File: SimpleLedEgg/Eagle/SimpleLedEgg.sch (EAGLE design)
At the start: 18 parts

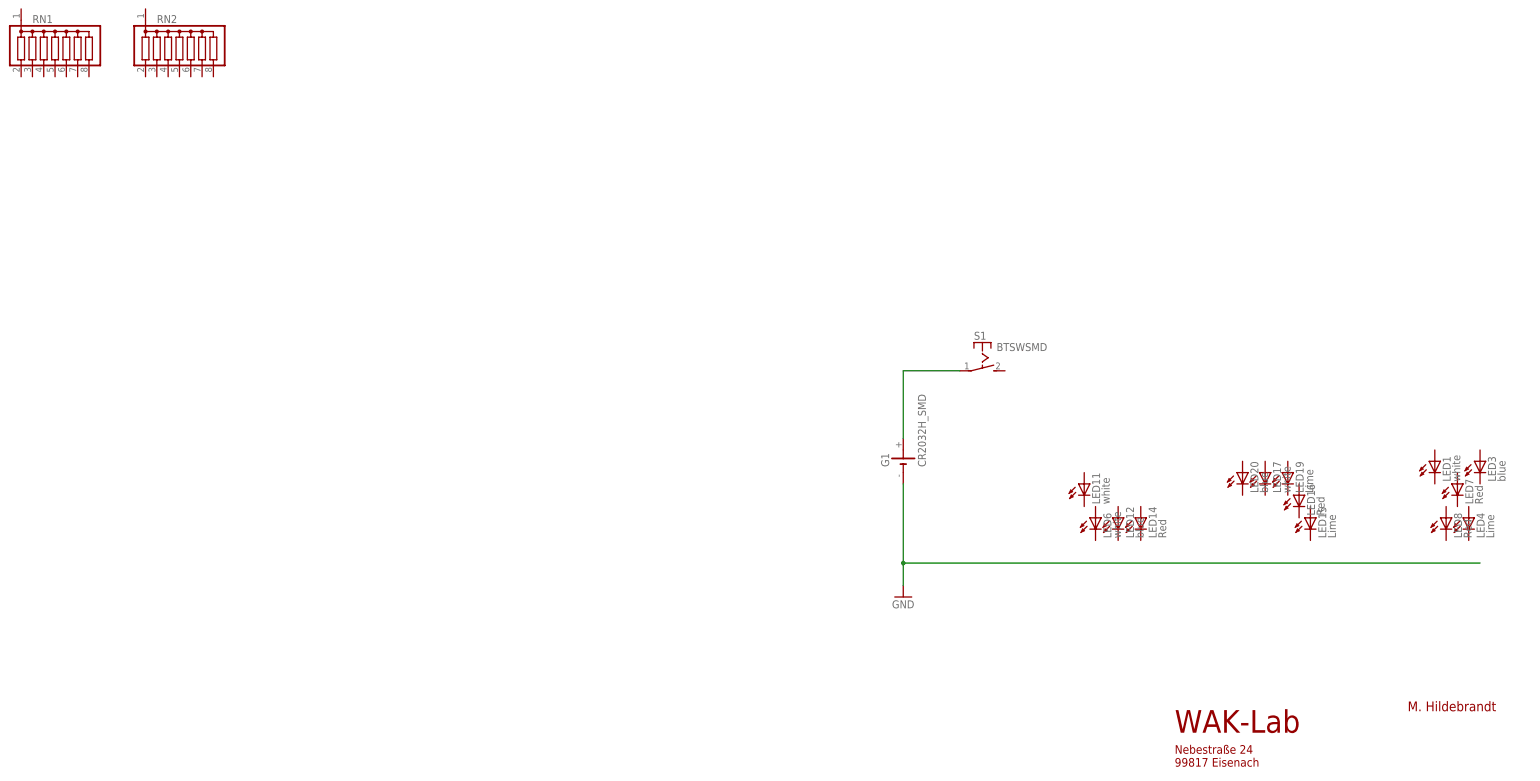
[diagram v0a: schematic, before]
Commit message: Gerber
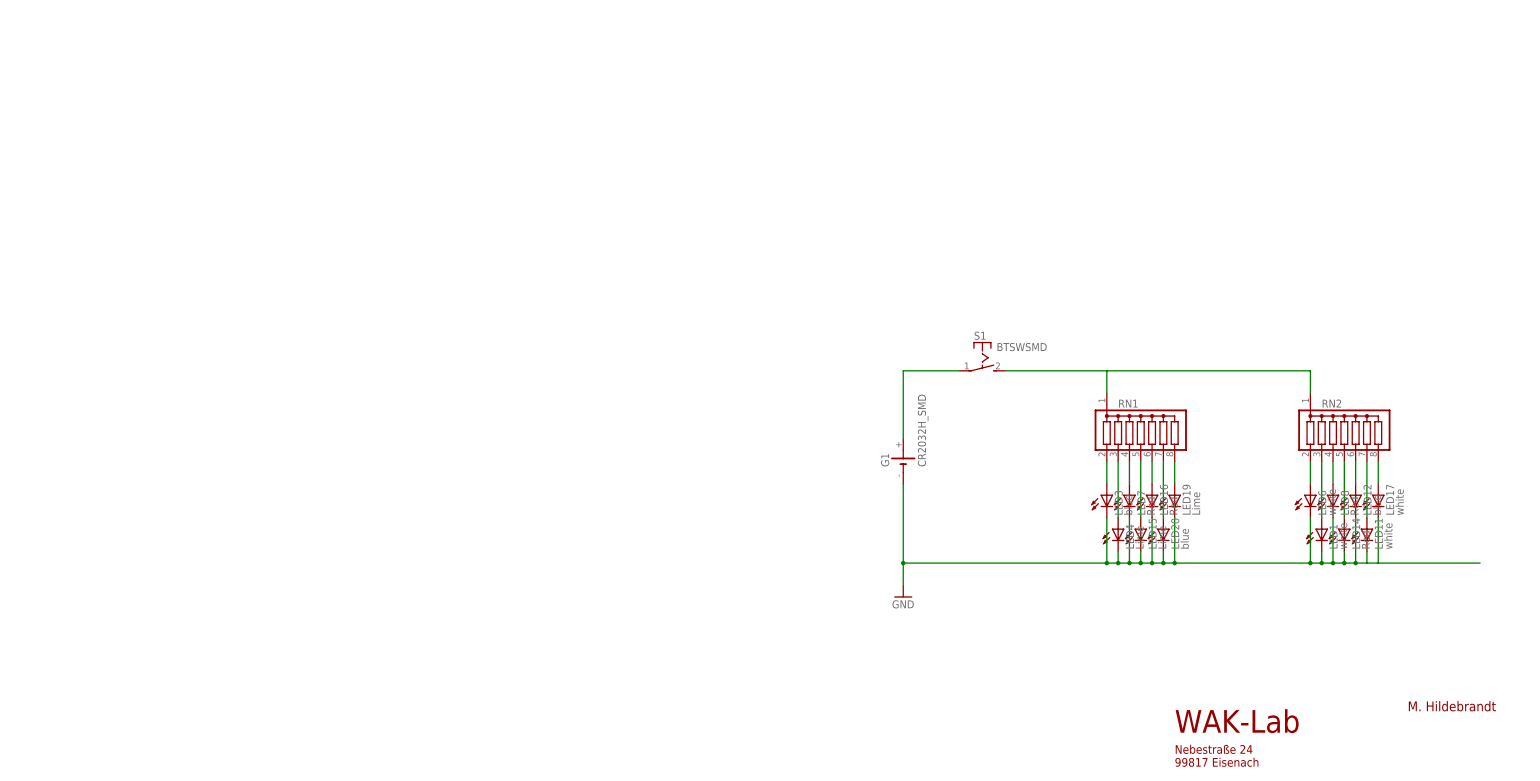
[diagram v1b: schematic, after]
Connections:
- new net N$1: RN1.1, RN2.1, S1.S
- new net N$10: LED1.A, RN2.3
- new net N$11: LED8.A, RN2.4
- new net N$12: LED12.A, RN2.6
- new net N$13: LED14.A, RN2.5
- new net N$14: LED11.A, RN2.7
- new net N$15: LED17.A, RN2.8
- new net N$2: LED3.A, RN1.2
- new net N$3: LED4.A, RN1.3
- new net N$4: LED7.A, RN1.4
- new net N$5: LED15.A, RN1.5
- new net N$6: LED16.A, RN1.6
- new net N$7: LED20.A, RN1.7
- new net N$8: LED19.A, RN1.8
- new net N$9: LED6.A, RN2.2
- net GND: now also LED1.C, LED11.C, LED12.C, LED14.C, LED15.C, LED16.C, LED17.C, LED19.C, LED20.C, LED3.C, LED4.C, LED6.C, LED7.C, LED8.C
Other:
- moved on the sheet: LED1, LED11, LED12, LED14, LED15, LED16, LED17, LED19, LED20, LED3, LED4, LED6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
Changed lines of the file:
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@@
 <sheet>
 <plain>
-<frame x1="-5.08" y1="-27.94" x2="271.78" y2="162.56" columns="8" rows="5" layer="94"/>
 <text x="448.564" y="-7.874" size="2.1844" layer="94">M. Hildebrandt</text>
 <text x="396.24" y="-12.7" size="5.08" layer="94">WAK-Lab</text>
@@
 </plain>
 <instances>
-<instance part="LED1" gate="G$1" x="454.66" y="48.26"/>
-<instance part="LED16" gate="G$1" x="424.18" y="40.64"/>
-<instance part="LED4" gate="G$1" x="462.28" y="35.56"/>
-<instance part="LED19" gate="G$1" x="421.64" y="45.72"/>
-<instance part="LED15" gate="G$1" x="426.72" y="35.56"/>
-<instance part="LED7" gate="G$1" x="459.74" y="43.18"/>
-<instance part="LED8" gate="G$1" x="457.2" y="35.56"/>
-<instance part="LED14" gate="G$1" x="388.62" y="35.56"/>
-<instance part="LED17" gate="G$1" x="416.56" y="45.72"/>
-<instance part="LED11" gate="G$1" x="375.92" y="43.18"/>
-<instance part="LED6" gate="G$1" x="378.46" y="35.56"/>
-<instance part="LED12" gate="G$1" x="383.54" y="35.56"/>
-<instance part="LED20" gate="G$1" x="411.48" y="45.72"/>
-<instance part="LED3" gate="G$1" x="464.82" y="48.26"/>
+<instance part="LED1" gate="G$1" x="429.26" y="33.02"/>
+<instance part="LED16" gate="G$1" x="391.16" y="40.64"/>
+<instance part="LED4" gate="G$1" x="383.54" y="33.02"/>
+<instance part="LED19" gate="G$1" x="396.24" y="40.64"/>
+<instance part="LED15" gate="G$1" x="388.62" y="33.02"/>
+<instance part="LED7" gate="G$1" x="386.08" y="40.64"/>
+<instance part="LED8" gate="G$1" x="431.8" y="40.64"/>
+<instance part="LED14" gate="G$1" x="434.34" y="33.02"/>
+<instance part="LED17" gate="G$1" x="441.96" y="40.64"/>
+<instance part="LED11" gate="G$1" x="439.42" y="33.02"/>
+<instance part="LED6" gate="G$1" x="426.72" y="40.64"/>
+<instance part="LED12" gate="G$1" x="436.88" y="40.64"/>
+<instance part="LED20" gate="G$1" x="393.7" y="33.02"/>
+<instance part="LED3" gate="G$1" x="381" y="40.64"/>
 <instance part="G1" gate="G$1" x="335.28" y="48.26" smashed="yes" rot="R90">
 <attribute name="NAME" x="332.105" y="46.99" size="1.778" layer="95" rot="R90"/>
@@
 <attribute name="SHEET" x="461.645" y="-22.86" size="2.54" layer="94"/>
 </instance>
-<instance part="RN1" gate="G$1" x="144.78" y="139.7"/>
-<instance part="RN2" gate="G$1" x="172.72" y="139.7"/>
+<instance part="RN1" gate="G$1" x="388.62" y="53.34"/>
+<instance part="RN2" gate="G$1" x="434.34" y="53.34"/>
 <instance part="S1" gate="G$1" x="353.06" y="68.58" rot="R270"/>
 </instances>
@@
 <pinref part="GND10" gate="1" pin="GND"/>
 <wire x1="335.28" y1="25.4" x2="335.28" y2="20.32" width="0.1524" layer="91"/>
-<wire x1="464.82" y1="25.4" x2="335.28" y2="25.4" width="0.1524" layer="91"/>
+<wire x1="464.82" y1="25.4" x2="441.96" y2="25.4" width="0.1524" layer="91"/>
 <junction x="335.28" y="25.4"/>
+<pinref part="LED3" gate="G$1" pin="C"/>
+<wire x1="441.96" y1="25.4" x2="439.42" y2="25.4" width="0.1524" layer="91"/>
+<wire x1="439.42" y1="25.4" x2="436.88" y2="25.4" width="0.1524" layer="91"/>
+<wire x1="436.88" y1="25.4" x2="434.34" y2="25.4" width="0.1524" layer="91"/>
+<wire x1="434.34" y1="25.4" x2="431.8" y2="25.4" width="0.1524" layer="91"/>
+<wire x1="431.8" y1="25.4" x2="429.26" y2="25.4" width="0.1524" layer="91"/>
+<wire x1="429.26" y1="25.4" x2="426.72" y2="25.4" width="0.1524" layer="91"/>
+<wire x1="426.72" y1="25.4" x2="396.24" y2="25.4" width="0.1524" layer="91"/>
+<wire x1="396.24" y1="25.4" x2="393.7" y2="25.4" width="0.1524" layer="91"/>
+<wire x1="393.7" y1="25.4" x2="391.16" y2="25.4" width="0.1524" layer="91"/>
+<wire x1="391.16" y1="25.4" x2="388.62" y2="25.4" width="0.1524" layer="91"/>
+<wire x1="388.62" y1="25.4" x2="386.08" y2="25.4" width="0.1524" layer="91"/>
+<wire x1="386.08" y1="25.4" x2="383.54" y2="25.4" width="0.1524" layer="91"/>
+<wire x1="383.54" y1="25.4" x2="381" y2="25.4" width="0.1524" layer="91"/>
+<wire x1="381" y1="25.4" x2="335.28" y2="25.4" width="0.1524" layer="91"/>
+<wire x1="381" y1="25.4" x2="381" y2="35.56" width="0.1524" layer="91"/>
+<junction x="381" y="25.4"/>
+<pinref part="LED4" gate="G$1" pin="C"/>
+<wire x1="383.54" y1="27.94" x2="383.54" y2="25.4" width="0.1524" layer="91"/>
+<junction x="383.54" y="25.4"/>
+<pinref part="LED7" gate="G$1" pin="C"/>
+<wire x1="386.08" y1="35.56" x2="386.08" y2="25.4" width="0.1524" layer="91"/>
+<junction x="386.08" y="25.4"/>
+<pinref part="LED19" gate="G$1" pin="C"/>
+<wire x1="396.24" y1="35.56" x2="396.24" y2="25.4" width="0.1524" layer="91"/>
+<pinref part="LED16" gate="G$1" pin="C"/>
+<wire x1="391.16" y1="35.56" x2="391.16" y2="25.4" width="0.1524" layer="91"/>
+<pinref part="LED15" gate="G$1" pin="C"/>
+<wire x1="388.62" y1="27.94" x2="388.62" y2="25.4" width="0.1524" layer="91"/>
+<junction x="388.62" y="25.4"/>
+<junction x="391.16" y="25.4"/>
+<junction x="396.24" y="25.4"/>
+<pinref part="LED20" gate="G$1" pin="C"/>
+<wire x1="393.7" y1="27.94" x2="393.7" y2="25.4" width="0.1524" layer="91"/>
+<junction x="393.7" y="25.4"/>
+<pinref part="LED6" gate="G$1" pin="C"/>
+<wire x1="426.72" y1="35.56" x2="426.72" y2="25.4" width="0.1524" layer="91"/>
+<junction x="426.72" y="25.4"/>
+<pinref part="LED1" gate="G$1" pin="C"/>
+<wire x1="429.26" y1="27.94" x2="429.26" y2="25.4" width="0.1524" layer="91"/>
+<junction x="429.26" y="25.4"/>
+<pinref part="LED8" gate="G$1" pin="C"/>
+<wire x1="431.8" y1="35.56" x2="431.8" y2="25.4" width="0.1524" layer="91"/>
+<junction x="431.8" y="25.4"/>
+<pinref part="LED14" gate="G$1" pin="C"/>
+<wire x1="434.34" y1="27.94" x2="434.34" y2="25.4" width="0.1524" layer="91"/>
+<junction x="434.34" y="25.4"/>
+<pinref part="LED12" gate="G$1" pin="C"/>
+<wire x1="436.88" y1="35.56" x2="436.88" y2="25.4" width="0.1524" layer="91"/>
+<junction x="436.88" y="25.4"/>
+<pinref part="LED11" gate="G$1" pin="C"/>
+<wire x1="439.42" y1="27.94" x2="439.42" y2="25.4" width="0.1524" layer="91"/>
+<pinref part="LED17" gate="G$1" pin="C"/>
+<wire x1="441.96" y1="35.56" x2="441.96" y2="25.4" width="0.1524" layer="91"/>
 </segment>
 </net>
@@
 </segment>
 </net>
+<net name="N$1" class="0">
+<segment>
+<pinref part="S1" gate="G$1" pin="S"/>
+<pinref part="RN1" gate="G$1" pin="1"/>
+<wire x1="358.14" y1="68.58" x2="381" y2="68.58" width="0.1524" layer="91"/>
+<wire x1="381" y1="68.58" x2="381" y2="63.5" width="0.1524" layer="91"/>
+<pinref part="RN2" gate="G$1" pin="1"/>
+<wire x1="381" y1="68.58" x2="426.72" y2="68.58" width="0.1524" layer="91"/>
+<wire x1="426.72" y1="68.58" x2="426.72" y2="63.5" width="0.1524" layer="91"/>
+</segment>
+</net>
+<net name="N$2" class="0">
+<segment>
+<pinref part="RN1" gate="G$1" pin="2"/>
+<pinref part="LED3" gate="G$1" pin="A"/>
+<wire x1="381" y1="43.18" x2="381" y2="48.26" width="0.1524" layer="91"/>
+</segment>
+</net>
+<net name="N$3" class="0">
+<segment>
+<pinref part="RN1" gate="G$1" pin="3"/>
+<pinref part="LED4" gate="G$1" pin="A"/>
+<wire x1="383.54" y1="48.26" x2="383.54" y2="35.56" width="0.1524" layer="91"/>
+</segment>
+</net>
+<net name="N$4" class="0">
+<segment>
+<pinref part="LED7" gate="G$1" pin="A"/>
+<pinref part="RN1" gate="G$1" pin="4"/>
+<wire x1="386.08" y1="43.18" x2="386.08" y2="48.26" width="0.1524" layer="91"/>
+</segment>
+</net>
+<net name="N$5" class="0">
+<segment>
+<pinref part="LED15" gate="G$1" pin="A"/>
+<pinref part="RN1" gate="G$1" pin="5"/>
+<wire x1="388.62" y1="35.56" x2="388.62" y2="48.26" width="0.1524" layer="91"/>
+</segment>
+</net>
+<net name="N$6" class="0">
+<segment>
+<pinref part="LED16" gate="G$1" pin="A"/>
+<pinref part="RN1" gate="G$1" pin="6"/>
+<wire x1="391.16" y1="43.18" x2="391.16" y2="48.26" width="0.1524" layer="91"/>
+</segment>
+</net>
+<net name="N$7" class="0">
+<segment>
+<pinref part="LED20" gate="G$1" pin="A"/>
+<pinref part="RN1" gate="G$1" pin="7"/>
+<wire x1="393.7" y1="35.56" x2="393.7" y2="48.26" width="0.1524" layer="91"/>
+</segment>
+</net>
+<net name="N$8" class="0">
+<segment>
+<pinref part="RN1" gate="G$1" pin="8"/>
+<pinref part="LED19" gate="G$1" pin="A"/>
+<wire x1="396.24" y1="48.26" x2="396.24" y2="43.18" width="0.1524" layer="91"/>
+</segment>
+</net>
+<net name="N$9" class="0">
+<segment>
+<pinref part="LED6" gate="G$1" pin="A"/>
+<pinref part="RN2" gate="G$1" pin="2"/>
+<wire x1="426.72" y1="43.18" x2="426.72" y2="48.26" width="0.1524" layer="91"/>
+</segment>
+</net>
+<net name="N$10" class="0">
+<segment>
+<pinref part="LED1" gate="G$1" pin="A"/>
+<pinref part="RN2" gate="G$1" pin="3"/>
+<wire x1="429.26" y1="35.56" x2="429.26" y2="48.26" width="0.1524" layer="91"/>
+</segment>
+</net>
+<net name="N$11" class="0">
+<segment>
+<pinref part="RN2" gate="G$1" pin="4"/>
+<pinref part="LED8" gate="G$1" pin="A"/>
+<wire x1="431.8" y1="43.18" x2="431.8" y2="48.26" width="0.1524" layer="91"/>
+</segment>
+</net>
+<net name="N$12" class="0">
+<segment>
+<pinref part="RN2" gate="G$1" pin="6"/>
+<pinref part="LED12" gate="G$1" pin="A"/>
+<wire x1="436.88" y1="43.18" x2="436.88" y2="48.26" width="0.1524" layer="91"/>
+</segment>
+</net>
+<net name="N$13" class="0">
+<segment>
+<pinref part="RN2" gate="G$1" pin="5"/>
+<pinref part="LED14" gate="G$1" pin="A"/>
+<wire x1="434.34" y1="35.56" x2="434.34" y2="48.26" width="0.1524" layer="91"/>
+</segment>
+</net>
+<net name="N$14" class="0">
+<segment>
+<pinref part="LED11" gate="G$1" pin="A"/>
+<pinref part="RN2" gate="G$1" pin="7"/>
+<wire x1="439.42" y1="35.56" x2="439.42" y2="48.26" width="0.1524" layer="91"/>
+</segment>
+</net>
+<net name="N$15" class="0">
+<segment>
+<pinref part="LED17" gate="G$1" pin="A"/>
+<pinref part="RN2" gate="G$1" pin="8"/>
+<wire x1="441.96" y1="43.18" x2="441.96" y2="48.26" width="0.1524" layer="91"/>
+</segment>
+</net>
